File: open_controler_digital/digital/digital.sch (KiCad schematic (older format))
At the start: 82 parts, among them J1 Conn_02x20_Odd_Even

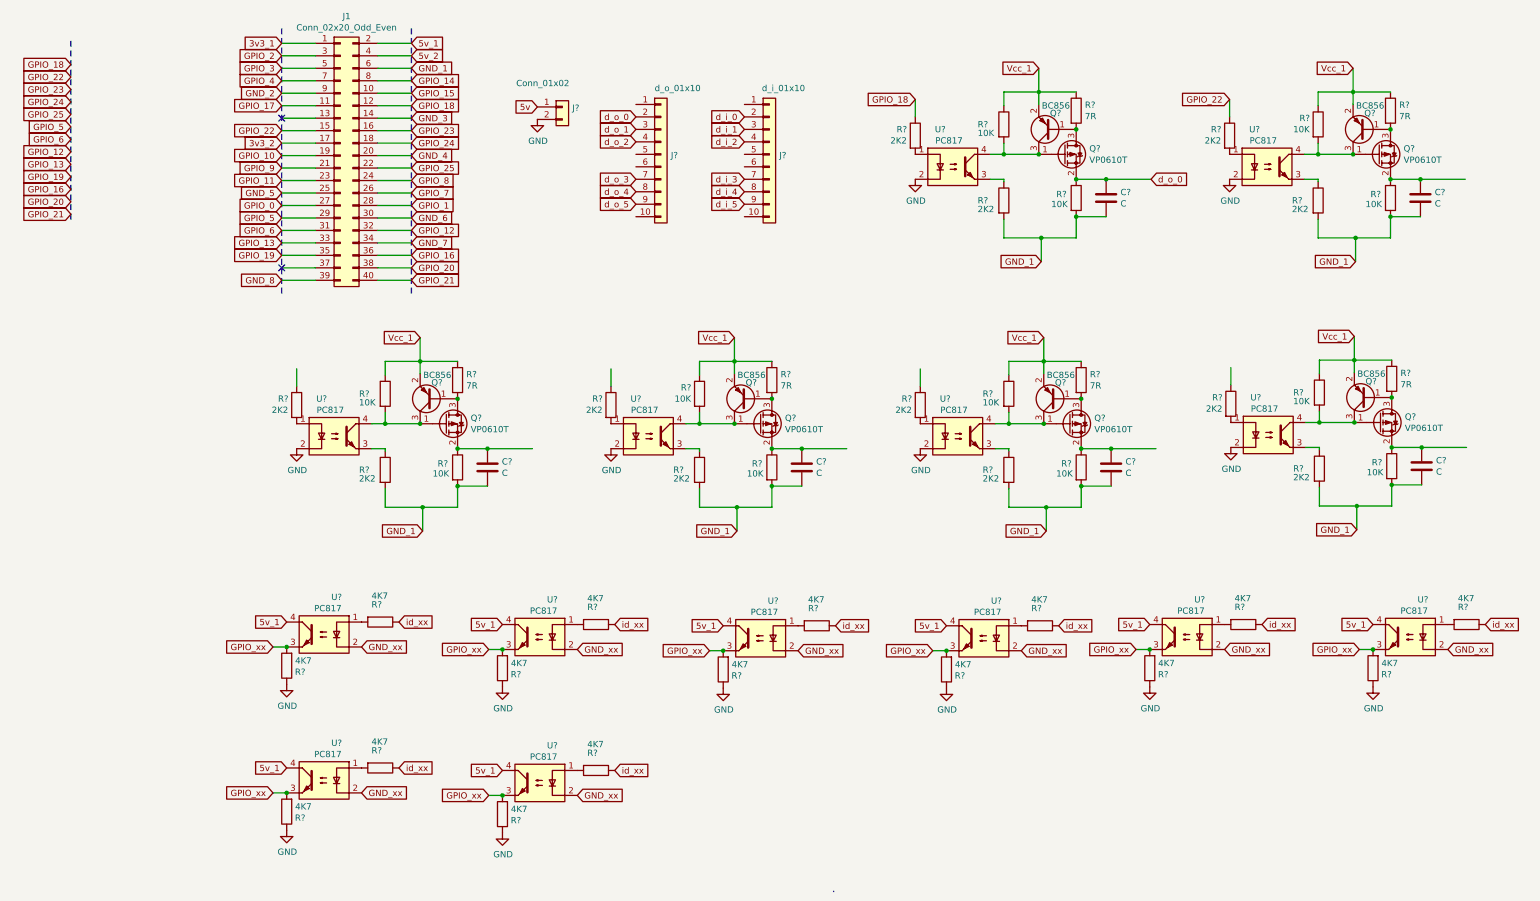
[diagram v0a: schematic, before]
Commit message: avances pcb digital
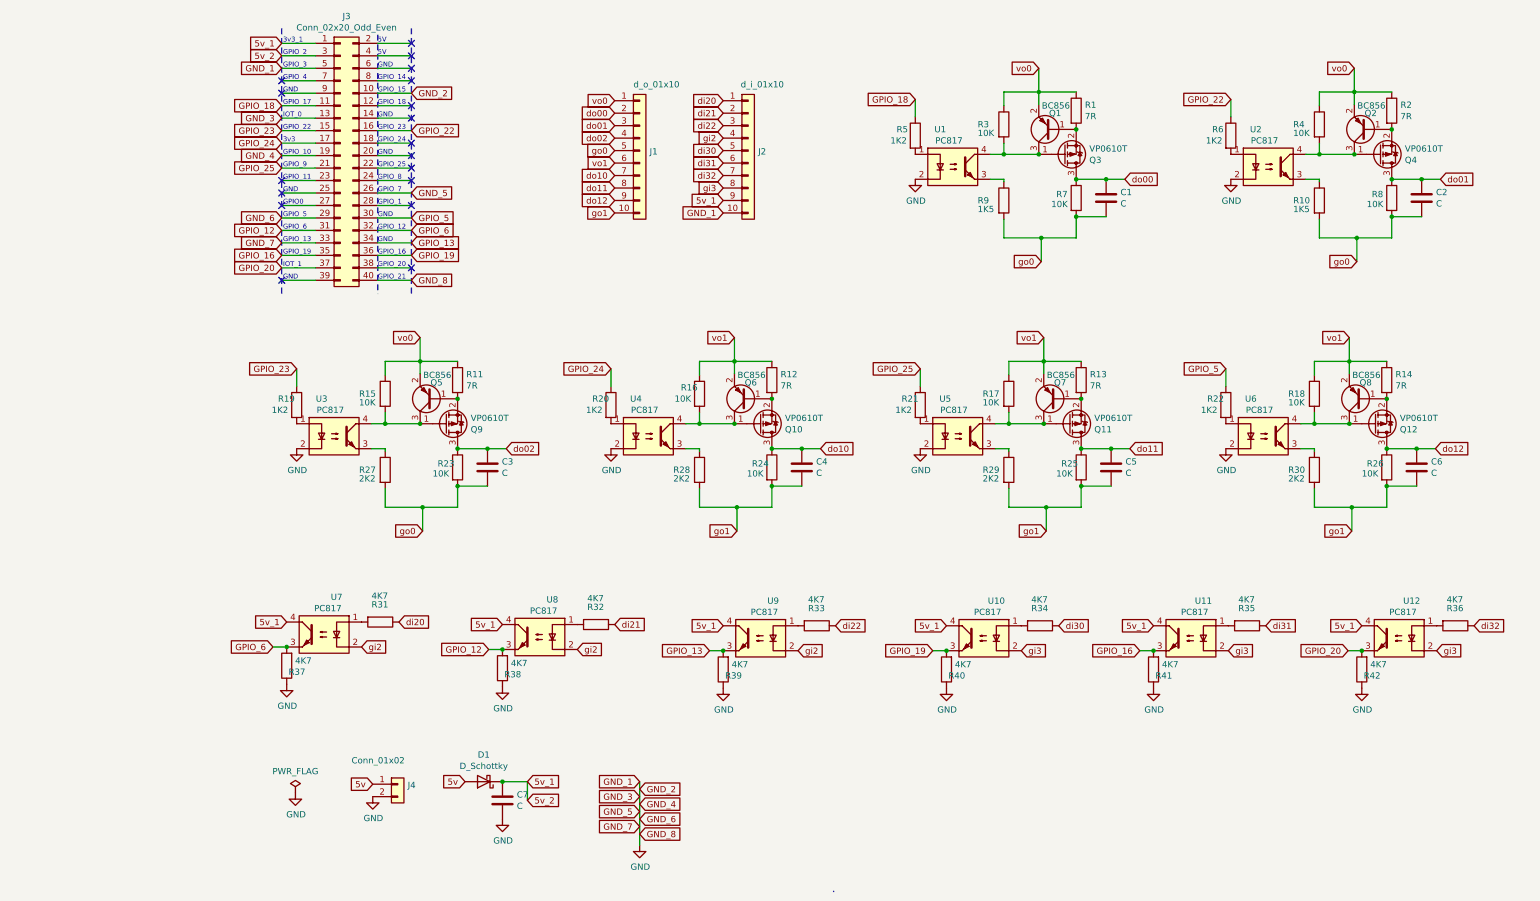
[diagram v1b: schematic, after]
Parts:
- removed C?: C, symbol Device:C
- removed Q?: BC856, Package_TO_SOT_SMD:SOT-23, symbol Transistor_BJT:BC856
- removed Q?: VP0610T, Package_TO_SOT_SMD:SOT-23, symbol Transistor_FET:VP0610T
- removed R? (x2): 10K, symbol Device:R
- removed R? (x2): 2K2, symbol Device:R
- removed R?: 7R, symbol Device:R
- removed R? (x6): 4K7, symbol Device:R
- removed U? (x4): PC817, Package_DIP:DIP-4_W7.62mm, symbol Isolator:PC817
- added C2, C7: C, Capacitor_SMD:C_1206_3216Metric_Pad1.42x1.75mm_HandSolder, symbol Device:C
- added D1: D_Schottky, Diode_SMD:D_2114_3652Metric, symbol Device:D_Schottky
- added Q2: BC856, Package_TO_SOT_SMD:SOT-23, symbol Transistor_BJT:BC856
- added Q4: VP0610T, Package_TO_SOT_SMD:SOT-23, symbol Transistor_FET:VP0610T
- added R10: 1K5, Resistor_SMD:R_1206_3216Metric_Pad1.42x1.75mm_HandSolder, symbol Device:R
- added R2: 7R, Resistor_SMD:R_1206_3216Metric_Pad1.42x1.75mm_HandSolder, symbol Device:R
- added R36, R42: 4K7, Resistor_SMD:R_1206_3216Metric_Pad1.42x1.75mm_HandSolder, symbol Device:R
- added R4, R8: 10K, Resistor_SMD:R_1206_3216Metric_Pad1.42x1.75mm_HandSolder, symbol Device:R
- added R6: 1K2, Resistor_SMD:R_1206_3216Metric_Pad1.42x1.75mm_HandSolder, symbol Device:R
- added U12, U2: PC817, Package_DIP:DIP-4_W8.89mm_SMDSocket_LongPads, symbol Isolator:PC817
- C1, C3, C4, C5, C6: renamed from C?; footprint (none) -> Capacitor_SMD:C_1206_3216Metric_Pad1.42x1.75mm_HandSolder
- J1, J2: renamed from J?; footprint (none) -> Connector_Phoenix_MC:PhoenixContact_MCV_1,5_10-G-3.5_1x10_P3.50mm_Vertical
- J4: renamed from J?; footprint (none) -> Connector_Phoenix_MC:PhoenixContact_MCV_1,5_2-G-3.5_1x02_P3.50mm_Vertical
- R1, R11, R12, R13, R14, R15, R16, R17, R18, R23, R24, R25, R26, R27, R28, R29, R3, R30, R31, R32, R33, R34, R35, R37, R38, R39, R40, R41, R7: renamed from R?; footprint (none) -> Resistor_SMD:R_1206_3216Metric_Pad1.42x1.75mm_HandSolder
- R19, R20, R21, R22, R5: renamed from R?; value 2K2 -> 1K2; footprint (none) -> Resistor_SMD:R_1206_3216Metric_Pad1.42x1.75mm_HandSolder
- R9: renamed from R?; value 2K2 -> 1K5; footprint (none) -> Resistor_SMD:R_1206_3216Metric_Pad1.42x1.75mm_HandSolder
- U1, U10, U11, U3, U4, U5, U6, U7, U8, U9: renamed from U?; footprint Package_DIP:DIP-4_W7.62mm -> Package_DIP:DIP-4_W8.89mm_SMDSocket_LongPads
- gave numbers to parts that had none: 10
- renumbered J1 to J3
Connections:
- net labels added: di20, di21, di22, di30, di31, di32, do00, do01, do02, do10, do11, do12, gi2, gi3, go0, go1, vo0, vo1
- net labels removed: 3v3_1, 3v3_2, GND_xx, GPIO_0, GPIO_1, GPIO_10, GPIO_11, GPIO_14, GPIO_15, GPIO_17, GPIO_2, GPIO_21, GPIO_3, GPIO_4, GPIO_7, GPIO_8, GPIO_9, GPIO_xx, Vcc_1, d_i_0, d_i_1, d_i_2, d_i_3, d_i_4, d_i_5, d_o_0, d_o_1, d_o_2, d_o_3, d_o_4, d_o_5, id_xx
- wire segments 168 -> 169
- no-connect marks 2 -> 18
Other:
- note added: "3v3"
- note added: "3v3_1"
- note added: "5V"
- note added: "GND"
- note added: "GPIO0"
- note added: "GPIO_1"
- note added: "GPIO_10"
- note added: "GPIO_11"
- note added: "GPIO_12"
- note added: "GPIO_13"
- note added: "GPIO_14"
- note added: "GPIO_15"
- note added: "GPIO_16"
- note added: "GPIO_17"
- note added: "GPIO_18"
- note added: "GPIO_19"
- note added: "GPIO_2"
- note added: "GPIO_20"
- note added: "GPIO_21"
- note added: "GPIO_22"
- note added: "GPIO_23"
- note added: "GPIO_24"
- note added: "GPIO_25"
- note added: "GPIO_3"
- note added: "GPIO_4"
- note added: "GPIO_5"
- note added: "GPIO_6"
- note added: "GPIO_7"
- note added: "GPIO_8"
- note added: "GPIO_9"
- note added: "IOT_0"
- note added: "IOT_1"
- moved on the sheet: C6, J1, J2, J4, Q12, Q8, R14, R18, R22, R26, R30, R35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
